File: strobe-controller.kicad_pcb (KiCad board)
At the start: 2 copper layers, 185 x 110 mm, 33 parts, among them J101 Power_in, J102 LED_R, J103 LED_G, J104 LED_W, J105 LED_B, J202 mono-jack, J302 mono-jack, J402 mono-jack, J502 mono-jack, Q105 BSP149, Q201 FQP30N06L, Q301 FQP30N06L, Q401 FQP30N06L, Q501 FQP30N06L

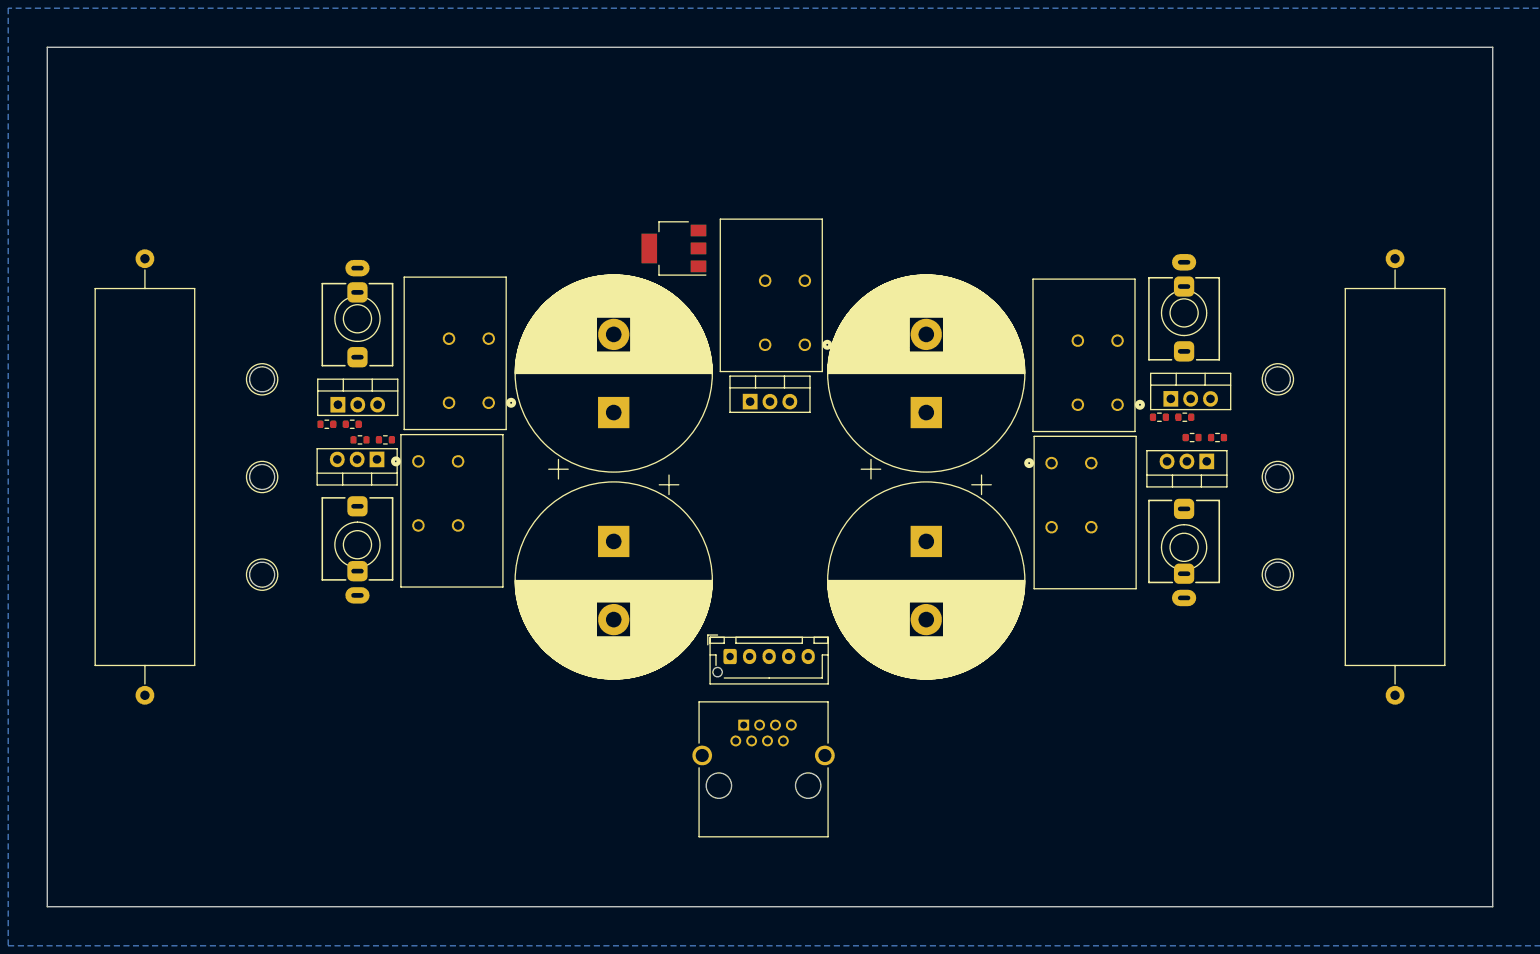
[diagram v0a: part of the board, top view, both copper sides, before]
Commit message: V1 for fab
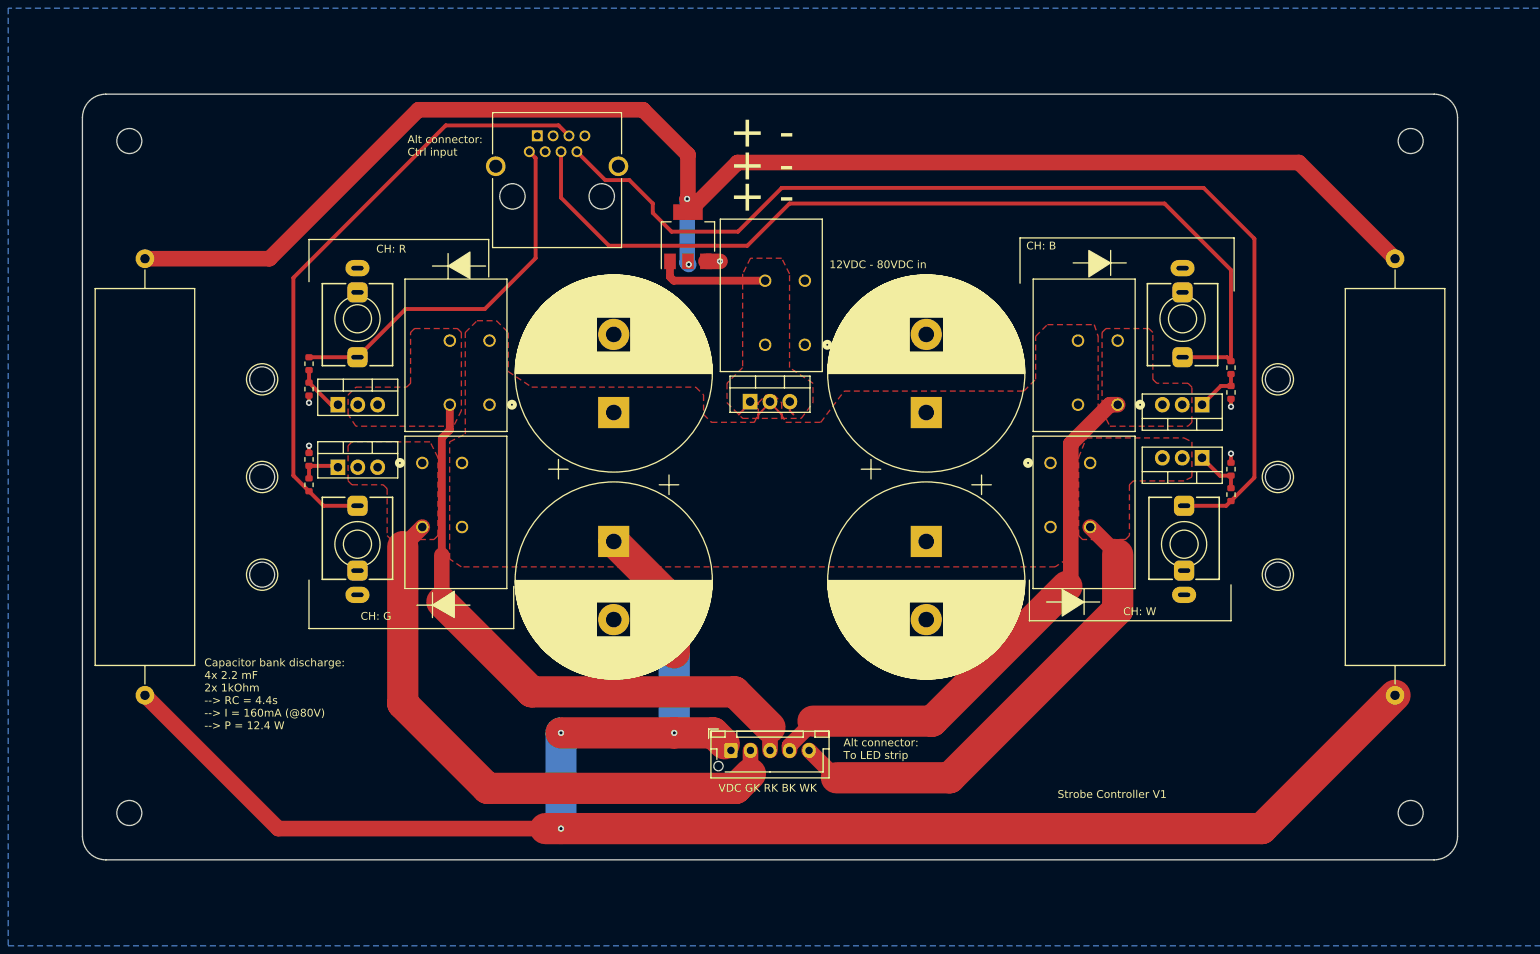
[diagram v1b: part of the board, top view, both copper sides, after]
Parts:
- added H103: MountingHole, MountingHole:MountingHole_3.2mm_M3_DIN965, F.Cu at (182.0, 57.0)
- added H104: MountingHole, MountingHole:MountingHole_3.2mm_M3_DIN965, F.Cu at (18.0, 57.0)
- added H105: MountingHole, MountingHole:MountingHole_3.2mm_M3_DIN965, F.Cu at (18.0, 143.0)
- added H106: MountingHole, MountingHole:MountingHole_3.2mm_M3_DIN965, F.Cu at (182.0, 143.0)
- J102: value LED_R -> LED_B
- J104: value LED_W -> LED_R
- J105: value LED_B -> LED_G
- moved CO101 79.9 mm to (72.8, 62.0)
- moved D101 12.0 mm to (95.0, 135.0)
- moved R201 11.1 mm to (159.0, 86.0), turned to -90 degrees
- moved R402 10.1 mm to (41.0, 97.8), turned to -90 degrees
- moved R401 8.70 mm to (41.0, 101.0), turned to 90 degrees
- moved R501 8.08 mm to (41.0, 85.5), turned to -90 degrees
- moved R301 7.50 mm to (159.0, 102.2), turned to 90 degrees
- moved R502 7.13 mm to (41.0, 88.8), turned to 90 degrees
- moved R202 6.71 mm to (159.0, 89.2), turned to 90 degrees
- moved R302 6.42 mm to (159.0, 99.0), turned to -90 degrees
- moved Q401 5.10 mm to (44.7, 98.8), turned to 0 degrees
- moved Q201 4.07 mm to (155.3, 90.8), turned to 180 degrees
- moved Q105 2.34 mm to (89.5, 69.2), turned to 90 degrees
- moved J202 0.78 mm to (152.8, 79.8)
- moved Q301 0.75 mm to (155.3, 97.5)
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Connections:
- CO101 pad Bl: LED_G -> LED_B
- CO101 pad Gr: LED_B -> LED_G
- D101 pad 1: drain_R -> VDC
- D101 pad 3: drain_B -> drain_R
- D101 pad 4: drain_W -> drain_B
- D101 pad 5: VDC -> drain_W
- J102 pad 1: drain_R -> drain_B
- J103 pad 2: drain_G -> drain_W
- J104 pad 2: drain_W -> drain_R
- J105 pad 1: drain_B -> drain_G
- J202 pad T: LED_R -> LED_B
- J302 pad T: LED_G -> LED_W
- J402 pad T: LED_B -> LED_G
- J502 pad T: LED_W -> LED_R
- Q201 pad 2: drain_R -> drain_B
- Q301 pad 2: drain_G -> drain_W
- Q401 pad 2: drain_B -> drain_G
- Q501 pad 2: drain_W -> drain_R
- R201 pad 1: LED_R -> LED_B
- R301 pad 1: LED_G -> LED_W
- R401 pad 1: LED_B -> LED_G
- R501 pad 1: LED_W -> LED_R
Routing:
- net VDC: track 0.00 -> 242.8 mm, vias 0 -> 4
- net Drain_shunt: track 0.00 -> 193.9 mm, vias 0 -> 2
- net LED_W: track 0.00 -> 137.7 mm
- net LED_B: track 0.00 -> 118.0 mm
- net drain_R: track 0.00 -> 81.8 mm
- net LED_G: track 0.00 -> 79.0 mm
- net drain_G: track 0.00 -> 76.4 mm
- net drain_B: track 0.00 -> 71.2 mm
- net drain_W: track 0.00 -> 61.9 mm
- net LED_R: track 0.00 -> 48.2 mm
- net Vin: track 0.00 -> 18.3 mm
- net Net-(Q501-G): track 0.00 -> 6.47 mm
- net Net-(Q301-G): track 0.00 -> 6.24 mm
- net Net-(Q201-G): track 0.00 -> 6.22 mm
- net GND: track 0.00 -> 5.82 mm, vias 0 -> 5
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- added copper zone on F.Cu, net VDC
- added copper zone on F.Cu, net Vin
- added copper zone on F.Cu, net drain_B
- added copper zone on F.Cu, net drain_G
- added copper zone on F.Cu, net drain_R
- added copper zone on F.Cu, net drain_W
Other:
- board size 185 x 110 mm -> 176 x 98 mm
- board text added: "+ -"
- board text added: "12VDC - 80VDC in"
- board text added: "Alt connector: Ctrl input"
- board text added: "Alt connector: To LED strip"
- board text added: "CH: B"
- board text added: "CH: G"
- board text added: "CH: R"
- board text added: "CH: W"
- board text added: "Capacitor bank discharge: 4x 2.2 mF 2x 1kOhm --> RC = 4.4s --> I = 160mA (@80V) --> P = 12.4 W"
- board text added: "Strobe Controller V1"
- board text added: "VDC GK RK BK WK"
